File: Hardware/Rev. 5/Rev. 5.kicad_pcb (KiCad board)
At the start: 4 copper layers, 29.2 x 29.2 mm, 28 parts, among them J1 Conn_01x03_Pin, J2 FFC_4_Pin, U1 MCP73831-2-OT, U3 W25Q128JVS, U4 AD7150, U5 PCC110

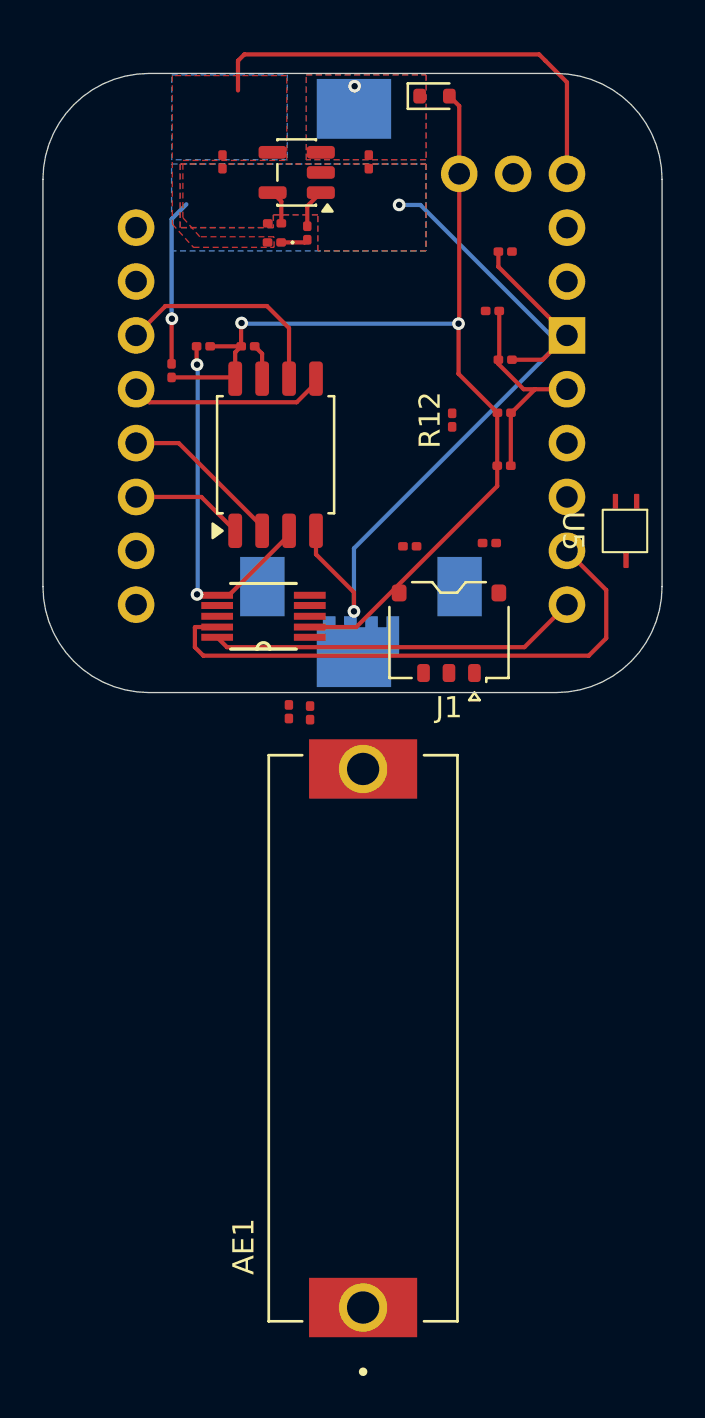
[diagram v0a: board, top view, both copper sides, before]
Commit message: Week 9 Changes
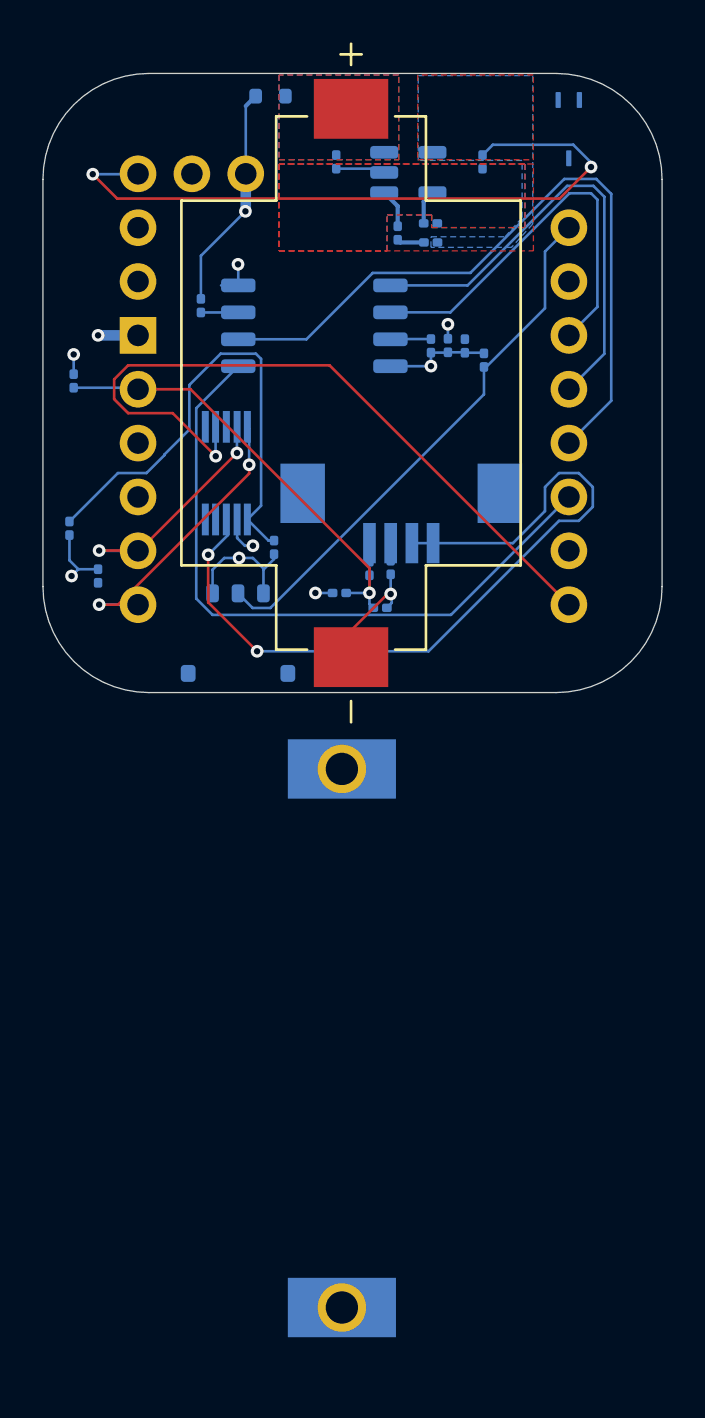
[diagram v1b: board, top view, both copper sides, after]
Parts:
- AE1, C1, C2, C3, C4, C5, D1, D2, J1, R1, R10, R11, R12, R2, R3, R4, R5, R6, R7, R8, R9, U1, U2, U3, U4, U5: moved to B.Cu
- BT1: moved to F.Cu
- moved U2 23.0 mm to (230.6, 74.2), turned to 180 degrees
- moved R7 20.4 mm to (205.9, 85.2), turned to -90 degrees
- moved U5 19.2 mm to (232.3, 73.3)
- moved R9 15.8 mm to (220.9, 94.0), turned to -90 degrees
- moved R11 14.8 mm to (207.1, 94.4), turned to 90 degrees
- moved C5 14.3 mm to (205.8, 92.2)
- moved R8 13.5 mm to (219.9, 94.0), turned to 90 degrees
- moved R10 13.1 mm to (220.4, 95.9)
- moved C4 13.1 mm to (223.6, 83.5)
- moved C1 12.3 mm to (225.2, 74.9)
- moved J1 9.95 mm to (213.7, 97.1)
- moved R6 9.81 mm to (218.5, 95.2)
- moved R5 9.37 mm to (224.4, 83.5), turned to -90 degrees
- moved R4 8.63 mm to (222.8, 83.5), turned to 90 degrees
- moved C3 7.78 mm to (215.4, 93.0)
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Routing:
- net FORCE+: track 0.00 -> 38.1 mm, vias 0 -> 2
- net 5/LPIO0: track 0.00 -> 34.6 mm, vias 0 -> 1
- net VBAT: track 48.6 -> 19.2 mm, vias 2 -> 5
- net GND: track 52.7 -> 24.0 mm, vias 3 -> 6
- net 6/CS: track 5.33 -> 32.0 mm
- net 8/COPI: track 7.78 -> 33.6 mm
- net 10/A0: track 0.00 -> 25.6 mm
- net Net-(U4-GND): track 0.00 -> 23.2 mm
- net Net-(U3-~{WP}/IO_{2}): track 17.2 -> 1.76 mm, vias 2 -> 0
- net 3/SCL1: track 26.8 -> 11.5 mm, vias 0 -> 2
- net 7/CIPO: track 9.52 -> 22.0 mm
- net 0/LPIO3: track 10.3 -> 21.4 mm, vias 0 -> 1
- net VIN: track 21.9 -> 32.6 mm, vias 0 -> 2
- net 9/SCLK: track 10.6 -> 19.2 mm
- net 4/SDA1: track 17.5 -> 13.7 mm, vias 0 -> 2
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- added copper zone on B.Cu, net GND
- added copper zone on F.Cu, net GND
- added copper zone on In1.Cu, net GND
- added copper zone on In2.Cu, net VBAT
- removed copper zone on B.Cu, net (none)
